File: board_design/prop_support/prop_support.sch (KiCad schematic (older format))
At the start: 15 parts, among them J1 Conn_02x03_Counter_Clockwise, SW1 SW_Push, U1 STM32F446RETx

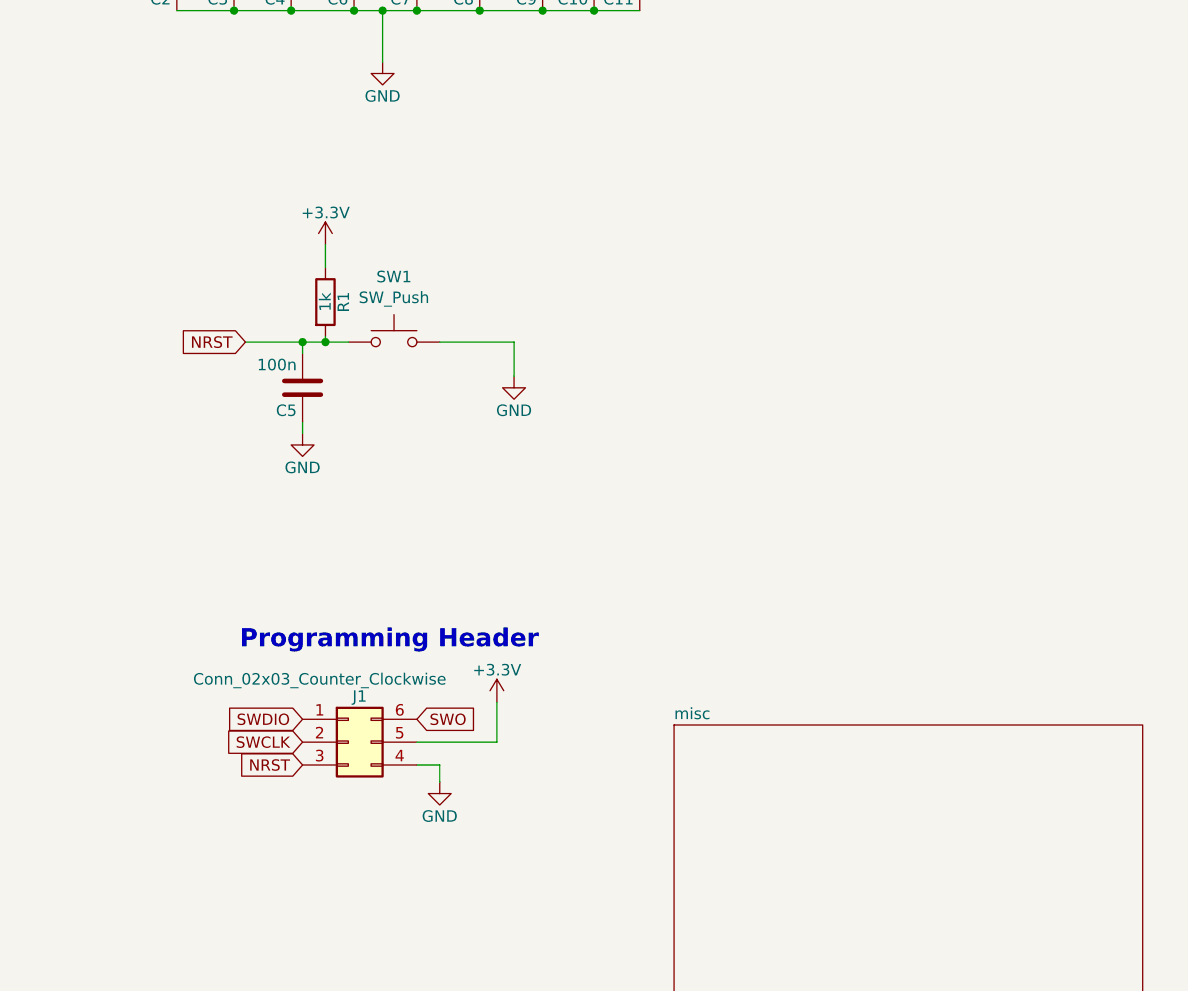
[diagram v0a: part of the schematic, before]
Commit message: first MX export
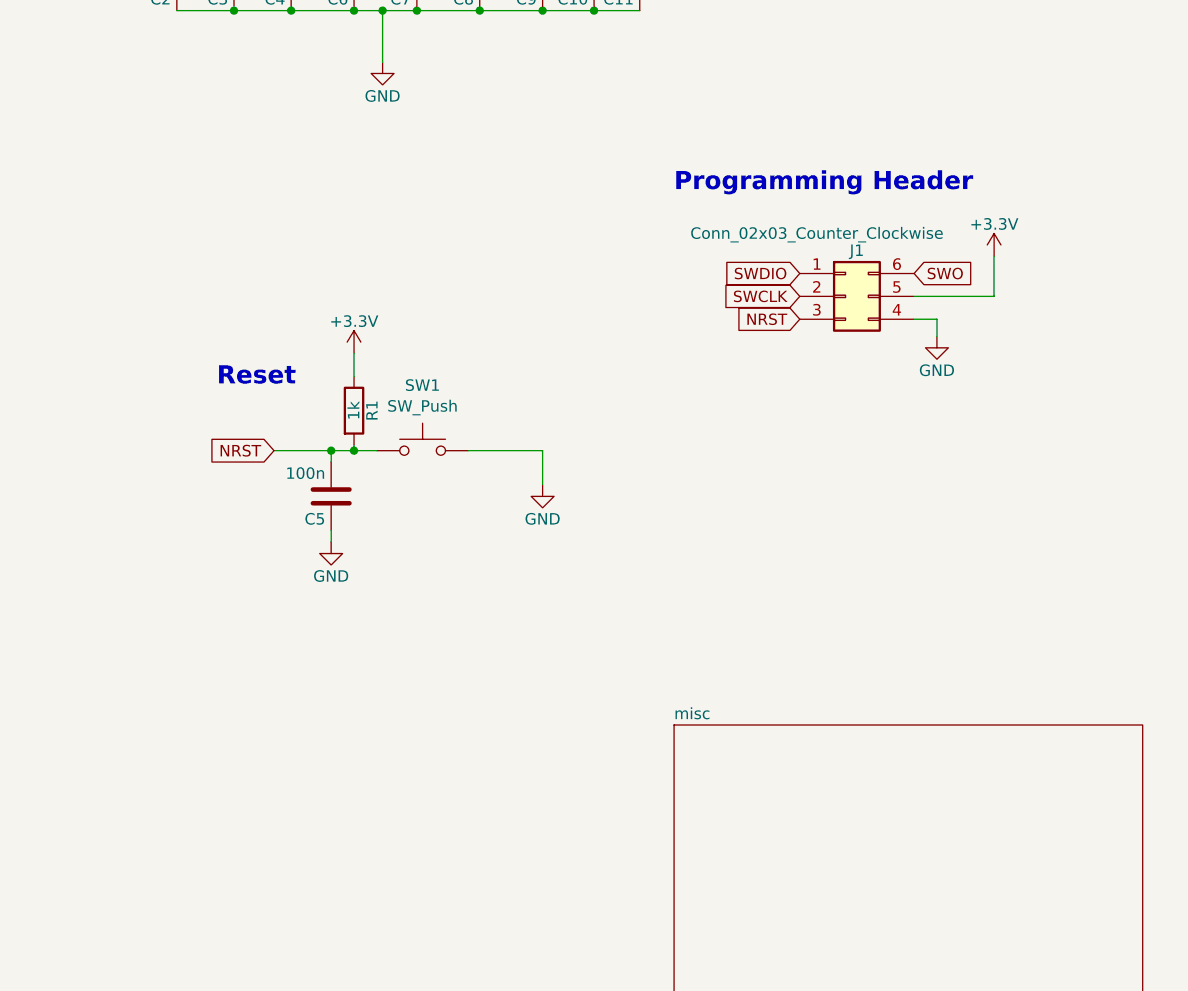
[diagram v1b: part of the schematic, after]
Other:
- note added: "Reset"
- moved on the sheet: C5, J1, R1, SW1
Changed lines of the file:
@@
 L power:GND #PWR0105
 U 1 1 5CA4278E
-P 5925 3525
-F 0 "#PWR0105" H 5925 3275 50  0001 C CNN
-F 1 "GND" H 5925 3375 50  0000 C CNN
-F 2 "" H 5925 3525 50  0001 C CNN
-F 3 "" H 5925 3525 50  0001 C CNN
-	1    5925 3525
+P 6050 4000
+F 0 "#PWR0105" H 6050 3750 50  0001 C CNN
+F 1 "GND" H 6050 3850 50  0000 C CNN
+F 2 "" H 6050 4000 50  0001 C CNN
+F 3 "" H 6050 4000 50  0001 C CNN
+	1    6050 4000
 	1    0    0    -1
 $EndComp
@@
 L Device:C C5
 U 1 1 5CA42795
-P 5000 3575
-F 0 "C5" H 5025 3675 50  0000 L CNN
-F 1 "100n" H 5025 3475 50  0000 L CNN
-F 2 "Capacitor_SMD:C_0805_2012Metric" H 5038 3425 50  0001 C CNN
-F 3 "" H 5000 3575 50  0001 C CNN
-	1    5000 3575
+P 5125 4050
+F 0 "C5" H 5150 4150 50  0000 L CNN
+F 1 "100n" H 5150 3950 50  0000 L CNN
+F 2 "Capacitor_SMD:C_0805_2012Metric" H 5163 3900 50  0001 C CNN
+F 3 "" H 5125 4050 50  0001 C CNN
+	1    5125 4050
 	-1   0    0    1
 $EndComp
@@
 L power:GND #PWR0106
 U 1 1 5CA4279B
-P 5000 3775
-F 0 "#PWR0106" H 5000 3525 50  0001 C CNN
-F 1 "GND" H 5000 3625 50  0000 C CNN
-F 2 "" H 5000 3775 50  0001 C CNN
-F 3 "" H 5000 3775 50  0001 C CNN
-	1    5000 3775
+P 5125 4250
+F 0 "#PWR0106" H 5125 4000 50  0001 C CNN
+F 1 "GND" H 5125 4100 50  0000 C CNN
+F 2 "" H 5125 4250 50  0001 C CNN
+F 3 "" H 5125 4250 50  0001 C CNN
+	1    5125 4250
 	1    0    0    -1
 $EndComp
@@
 $EndComp
 Wire Wire Line
-	5600 3375 5925 3375
-Wire Wire Line
-	5925 3375 5925 3525
-Wire Wire Line
-	4750 3375 5000 3375
-Wire Wire Line
-	5000 3425 5000 3375
-Connection ~ 5000 3375
-Wire Wire Line
-	5000 3725 5000 3775
+	5725 3850 6050 3850
+Wire Wire Line
+	6050 3850 6050 4000
+Wire Wire Line
+	4875 3850 5125 3850
+Wire Wire Line
+	5125 3900 5125 3850
+Connection ~ 5125 3850
+Wire Wire Line
+	5125 4200 5125 4250
 Wire Wire Line
 	4450 1625 4700 1625
@@
 L Device:R R1
 U 1 1 5CA427FD
-P 5100 3200
-F 0 "R1" V 5180 3200 50  0000 C CNN
-F 1 "1k" V 5100 3200 50  0000 C CNN
-F 2 "Resistor_SMD:R_0805_2012Metric" V 5030 3200 50  0001 C CNN
-F 3 "" H 5100 3200 50  0001 C CNN
-	1    5100 3200
+P 5225 3675
+F 0 "R1" V 5305 3675 50  0000 C CNN
+F 1 "1k" V 5225 3675 50  0000 C CNN
+F 2 "Resistor_SMD:R_0805_2012Metric" V 5155 3675 50  0001 C CNN
+F 3 "" H 5225 3675 50  0001 C CNN
+	1    5225 3675
 	1    0    0    -1
 $EndComp
@@
 L power:+3.3V #PWR0109
 U 1 1 5CA42803
-P 5100 2950
-F 0 "#PWR0109" H 5100 2800 50  0001 C CNN
-F 1 "+3.3V" H 5100 3090 50  0000 C CNN
-F 2 "" H 5100 2950 50  0001 C CNN
-F 3 "" H 5100 2950 50  0001 C CNN
-	1    5100 2950
-	1    0    0    -1
-$EndComp
-Wire Wire Line
-	5100 2950 5100 3050
-Wire Wire Line
-	5100 3350 5100 3375
-Connection ~ 5100 3375
-Wire Wire Line
-	5000 3375 5100 3375
+P 5225 3425
+F 0 "#PWR0109" H 5225 3275 50  0001 C CNN
+F 1 "+3.3V" H 5225 3565 50  0000 C CNN
+F 2 "" H 5225 3425 50  0001 C CNN
+F 3 "" H 5225 3425 50  0001 C CNN
+	1    5225 3425
+	1    0    0    -1
+$EndComp
+Wire Wire Line
+	5225 3425 5225 3525
+Wire Wire Line
+	5225 3825 5225 3850
+Connection ~ 5225 3850
+Wire Wire Line
+	5125 3850 5225 3850
 Wire Wire Line
 	4700 1625 4950 1625
@@
 	5350 1925 5500 1925
 Wire Wire Line
-	5100 3375 5200 3375
-Text GLabel 5000 5025 0    49   Input ~ 0
+	5225 3850 5325 3850
+Text GLabel 7175 3075 0    49   Input ~ 0
 SWDIO
-Text GLabel 5000 5125 0    49   Input ~ 0
+Text GLabel 7175 3175 0    49   Input ~ 0
 SWCLK
-Text GLabel 5500 5025 2    49   Input ~ 0
+Text GLabel 7675 3075 2    49   Input ~ 0
 SWO
-Text GLabel 5000 5225 0    49   Input ~ 0
+Text GLabel 7175 3275 0    49   Input ~ 0
 NRST
 $Comp
 L power:+3.3V #PWR0110
 U 1 1 5CA42822
-P 5850 4950
-F 0 "#PWR0110" H 5850 4800 50  0001 C CNN
-F 1 "+3.3V" H 5850 5090 50  0000 C CNN
-F 2 "" H 5850 4950 50  0001 C CNN
-F 3 "" H 5850 4950 50  0001 C CNN
-	1    5850 4950
+P 8025 3000
+F 0 "#PWR0110" H 8025 2850 50  0001 C CNN
+F 1 "+3.3V" H 8025 3140 50  0000 C CNN
+F 2 "" H 8025 3000 50  0001 C CNN
+F 3 "" H 8025 3000 50  0001 C CNN
+	1    8025 3000
 	1    0    0    -1
 $EndComp
@@
 L power:GND #PWR0111
 U 1 1 5CA42828
-P 5600 5300
-F 0 "#PWR0111" H 5600 5050 50  0001 C CNN
-F 1 "GND" H 5600 5150 50  0000 C CNN
-F 2 "" H 5600 5300 50  0001 C CNN
-F 3 "" H 5600 5300 50  0001 C CNN
-	1    5600 5300
-	1    0    0    -1
-$EndComp
-Text Notes 4725 4725 0    79   ~ 16
+P 7775 3350
+F 0 "#PWR0111" H 7775 3100 50  0001 C CNN
+F 1 "GND" H 7775 3200 50  0000 C CNN
+F 2 "" H 7775 3350 50  0001 C CNN
+F 3 "" H 7775 3350 50  0001 C CNN
+	1    7775 3350
+	1    0    0    -1
+$EndComp
+Text Notes 6625 2725 0    79   ~ 16
 Programming Header
 Wire Wire Line
-	5850 4950 5850 5125
-Wire Wire Line
-	5850 5125 5500 5125
-Wire Wire Line
-	5500 5225 5600 5225
-Wire Wire Line
-	5600 5225 5600 5300
+	8025 3000 8025 3175
+Wire Wire Line
+	8025 3175 7675 3175
+Wire Wire Line
+	7675 3275 7775 3275
+Wire Wire Line
+	7775 3275 7775 3350
 $Comp
 L Connector_Generic:Conn_02x03_Counter_Clockwise J1
 U 1 1 5CA42833
-P 5200 5125
-F 0 "J1" H 5250 5325 50  0000 C CNN
-F 1 "Conn_02x03_Counter_Clockwise" H 5075 5400 50  0000 C CNN
-F 2 "Connector_PinHeader_2.54mm:PinHeader_2x03_P2.54mm_Vertical" H 5200 5125 50  0001 C CNN
-F 3 "" H 5200 5125 50  0001 C CNN
-	1    5200 5125
+P 7375 3175
+F 0 "J1" H 7425 3375 50  0000 C CNN
+F 1 "Conn_02x03_Counter_Clockwise" H 7250 3450 50  0000 C CNN
+F 2 "Connector_PinHeader_2.54mm:PinHeader_2x03_P2.54mm_Vertical" H 7375 3175 50  0001 C CNN
+F 3 "" H 7375 3175 50  0001 C CNN
+	1    7375 3175
 	1    0    0    -1
 $EndComp
@@
 Text GLabel 1750 4100 0    50   Input ~ 0
 en_vlv7
-Text GLabel 4750 3375 0    50   Input ~ 0
+Text GLabel 4875 3850 0    50   Input ~ 0
 NRST
 Text GLabel 3150 4200 2    50   Input ~ 0
@@
 L Switch:SW_Push SW1
 U 1 1 5CA14A08
-P 5400 3375
-F 0 "SW1" H 5400 3660 50  0000 C CNN
-F 1 "SW_Push" H 5400 3569 50  0000 C CNN
-F 2 "davenport_kicad_footprints:SKQGADE010" H 5400 3575 50  0001 C CNN
-F 3 "~" H 5400 3575 50  0001 C CNN
-	1    5400 3375
+P 5525 3850
+F 0 "SW1" H 5525 4135 50  0000 C CNN
+F 1 "SW_Push" H 5525 4044 50  0000 C CNN
+F 2 "davenport_kicad_footprints:SKQGADE010" H 5525 4050 50  0001 C CNN
+F 3 "~" H 5525 4050 50  0001 C CNN
+	1    5525 3850
 	1    0    0    -1
 $EndComp
@@
 NoConn ~ 1750 3800
 NoConn ~ 1750 3300
+Text Notes 4625 3575 0    79   ~ 16
+Reset
 $EndSCHEMATC
